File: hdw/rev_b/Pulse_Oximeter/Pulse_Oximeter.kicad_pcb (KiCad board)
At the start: 4 copper layers, 100 x 83 mm, 287 parts, among them J1201 USB_B_Mini, J1202 OSEPP_FTDI_01, J201 +12V IN, J801 PICKIT4, Q401 BSS214NW, Q402 BSS214NW, Q801 BSS214NW, SW1701 Cap_Touch, SW801 MRST, U1101 PIC32MZ0512EFE064T-I_PT, U1201 TLV6700, U1202 FT234XD, U1203 TXB0102DCU, U1204 TPD3S014DBVR, U1301 INA219BxDCN, U1302 MCP9804, U1401 DS1683, U1501 TPS22929D, U1502 TCA9803, U1503 MAX30102, U1504 74LVC1G97, U1601 74LVC1G97, U1602 Generic 20x04 LCD, U1701 AT42QT1010-TSHR, U1702 74LVC1G97, U1801 74LVC1G97, U1802 74LVC1G97, U1803 74LVC1G97, U1804 74LVC1G97, U1901 74LVC1G97, U1902 74LVC1G97, U1903 74LVC1G97, U1904 74LVC1G97, U2001 MCP9804, U2002 LTC1694, U201 TPS26600RHFT, U301 INA219BxDCN, U302 MCP9804, U401 74LVC1G97, U402 TPS62152, U501 MCP9804, U502 INA219BxDCN, U601 TPS7A7200RGTR, U701 MCP9804, U702 INA219BxDCN, X1001 ASE-8.000MHz

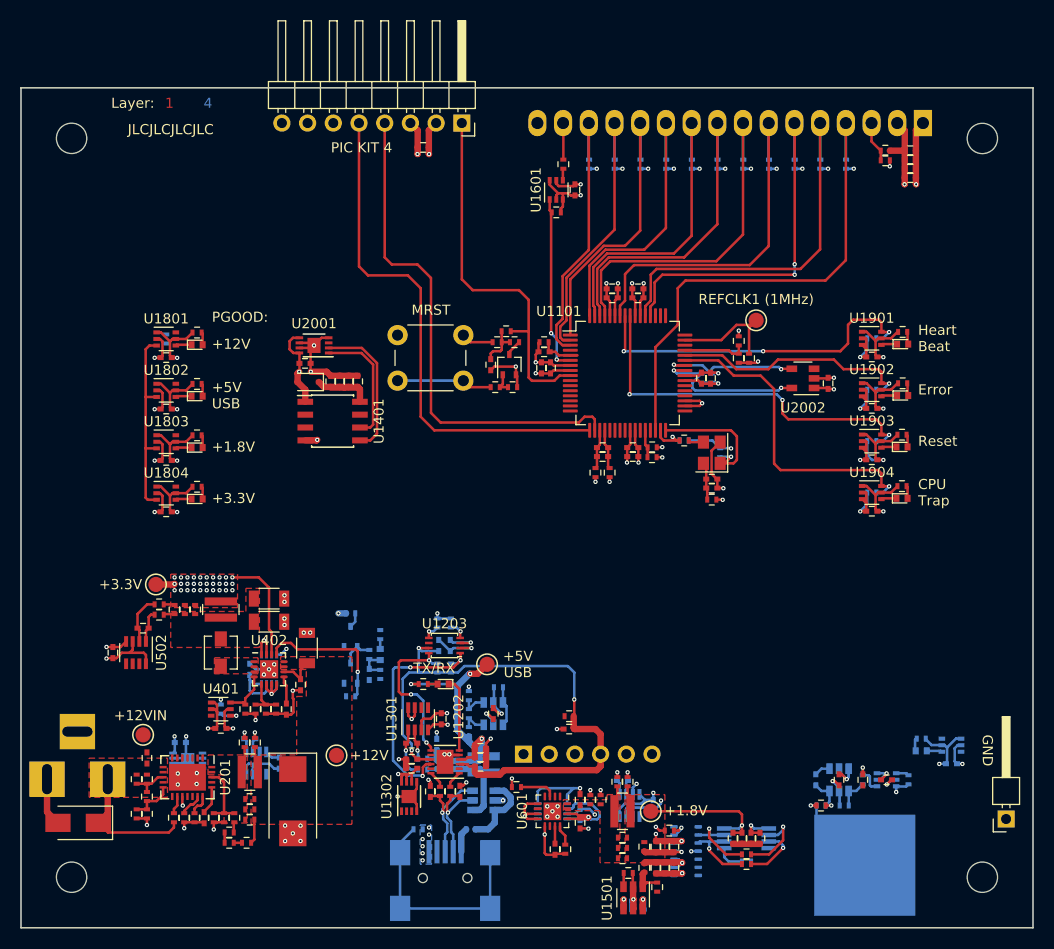
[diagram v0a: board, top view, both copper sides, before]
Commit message: got everything connected
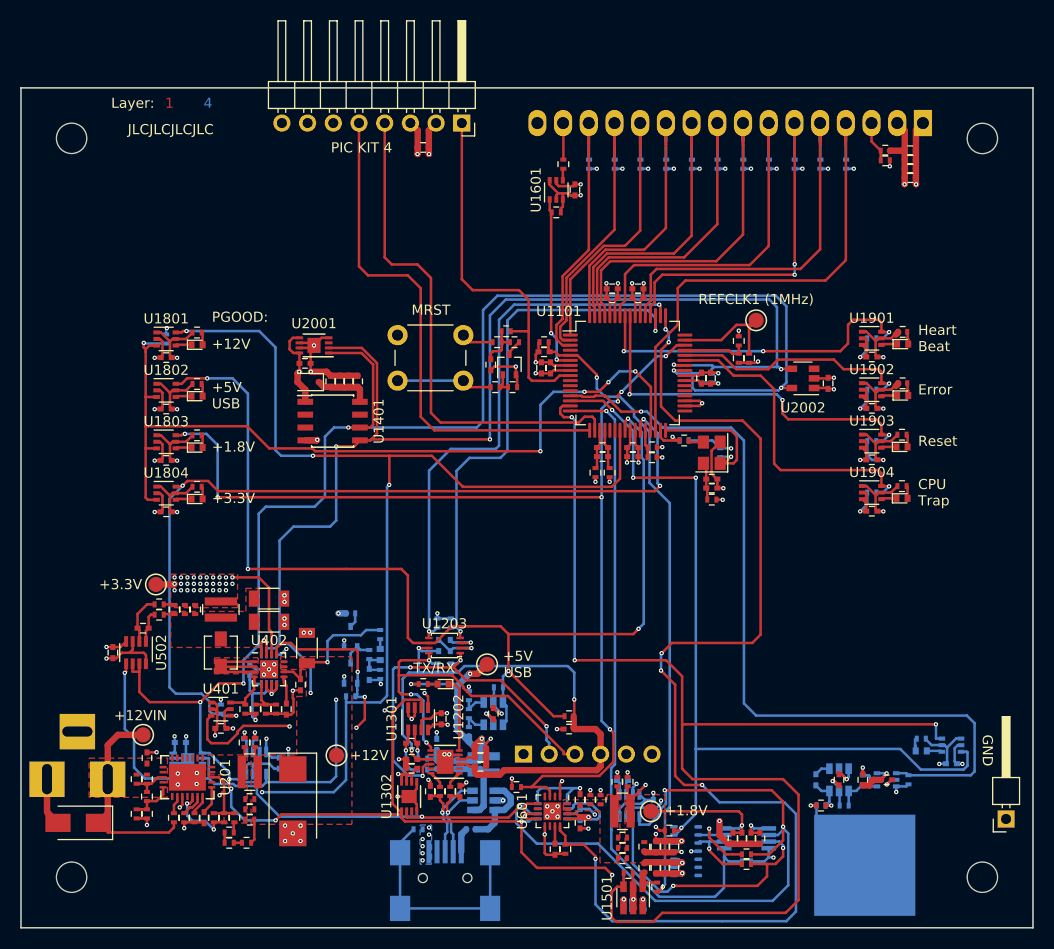
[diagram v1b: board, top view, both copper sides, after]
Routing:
- net I2C_SCL: track 35.1 -> 278.1 mm, vias 3 -> 13
- net I2C_SDA: track 33.6 -> 252.3 mm, vias 3 -> 12
- net POS3P3_POX_Enable: track 1.36 -> 122.3 mm, vias 0 -> 3
- net POS1P8_RUN: track 2.05 -> 117.5 mm, vias 0 -> 6
- net POS12_PGOOD: track 6.49 -> 118.0 mm, vias 0 -> 5
- net POS5_USB_PGOOD: track 3.99 -> 111.5 mm, vias 0 -> 5
- net POS1P8_PGOOD: track 3.57 -> 107.0 mm, vias 0 -> 7
- net POS3P3_PGOOD: track 2.19 -> 86.6 mm, vias 1 -> 4
- net ~POX_INT: track 1.96 -> 85.2 mm, vias 1 -> 4
- net Cap_Touch_Power: track 1.29 -> 81.4 mm, vias 0 -> 1
- net PGOOD_LED_SHDN: track 19.2 -> 84.0 mm, vias 0 -> 5
- net POX_I2C_Enable: track 2.81 -> 66.8 mm, vias 0 -> 1
- net POS3P3_POX_ADC: track 3.89 -> 62.1 mm, vias 0 -> 2
- net USB_UART_RX: track 1.64 -> 55.5 mm, vias 1 -> 2
- net USB_UART_TX: track 1.77 -> 54.3 mm, vias 1 -> 2
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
